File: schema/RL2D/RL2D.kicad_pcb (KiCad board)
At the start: 2 copper layers, 9 parts, among them J1 Steer_Joystick, SW1 SW_FancyButton, SW2 SW_FancyButton, SW3 SW_FancyButton, SW4 SW_On, U1 ILI9341 2.8" TFT LCD

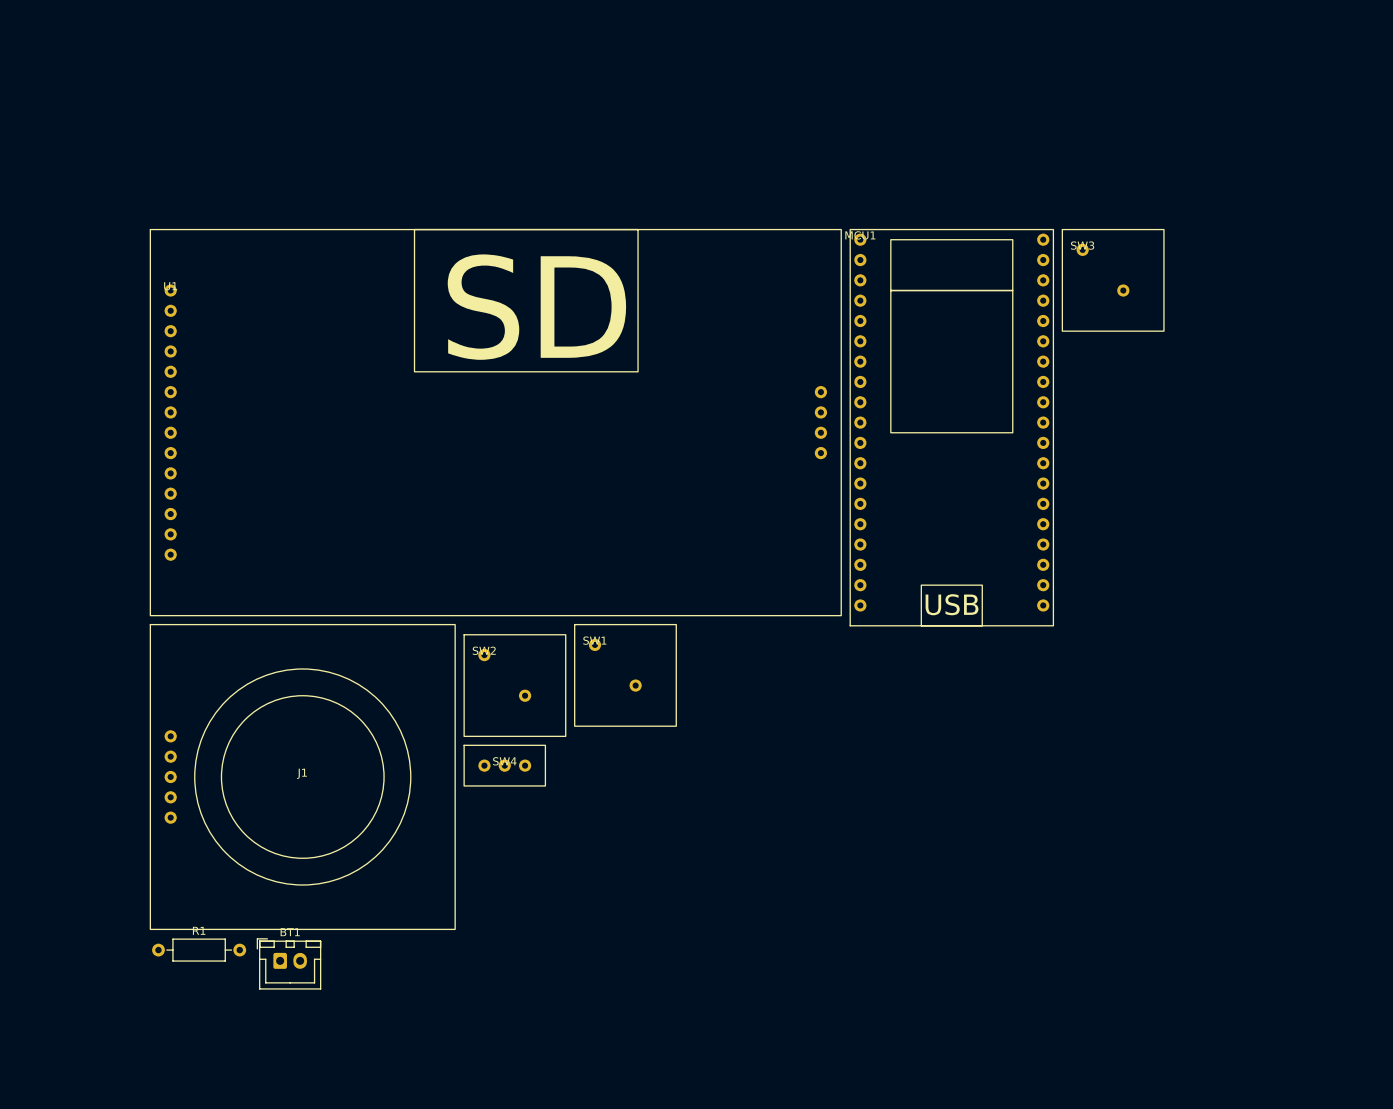
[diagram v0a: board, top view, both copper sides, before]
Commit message: newpcb
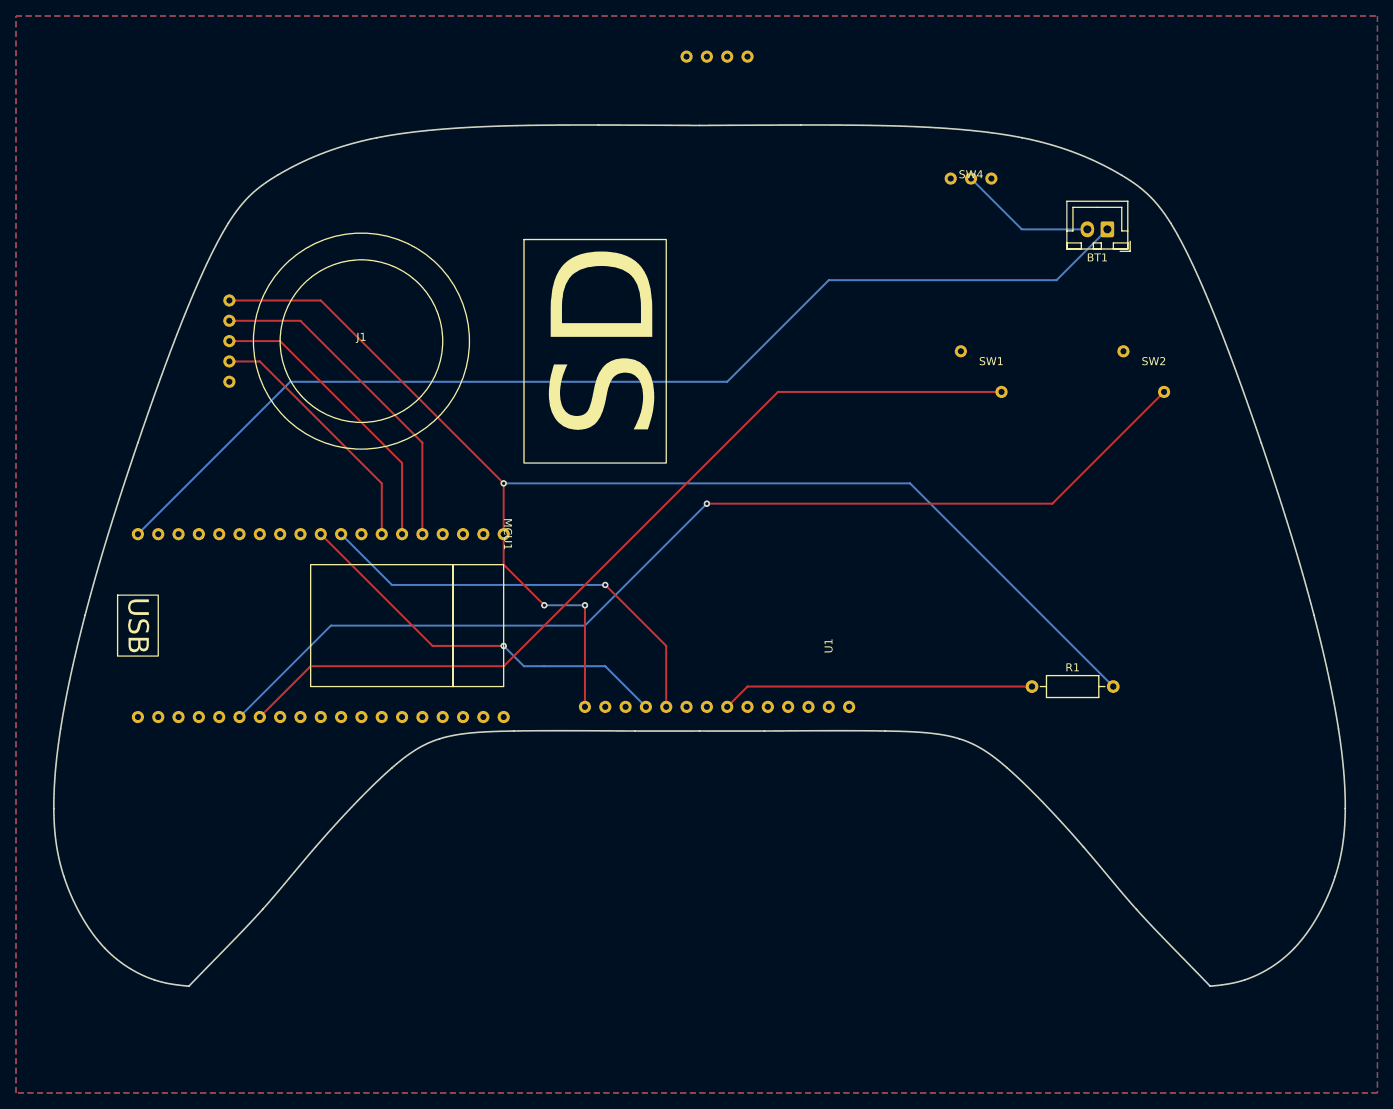
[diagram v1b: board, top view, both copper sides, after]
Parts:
- removed SW3: SW_FancyButton, RL2D:FancyButton
- SW1: value SW_FancyButton -> Brake Button
- SW2: value SW_FancyButton -> Accel Button
- SW4: value SW_On -> On Switch
- moved BT1 138.0 mm to (197.4, 47.0), turned to 180 degrees
- moved R1 114.1 mm to (188.0, 104.1)
- moved SW4 93.7 mm to (180.3, 40.6)
- moved SW2 88.4 mm to (199.4, 62.2)
- moved U1 73.4 mm to (132.1, 106.7), turned to 90 degrees
- moved SW1 58.6 mm to (179.1, 62.2)
- moved MCU1 57.8 mm to (121.9, 85.1), turned to -90 degrees
- moved J1 55.0 mm to (104.1, 61.0)
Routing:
- net +3V3: track 0.00 -> 165.6 mm, vias 0 -> 3
- net VDC: track 0.00 -> 137.0 mm
- net Net-(MCU1-Pad25): track 0.00 -> 132.4 mm, vias 0 -> 1
- net Net-(MCU1-Pad26): track 0.00 -> 109.5 mm
- net Net-(MCU1-Pad9): track 0.00 -> 54.0 mm, vias 0 -> 1
- net Net-(MCU1-Pad10): track 0.00 -> 49.6 mm, vias 0 -> 1
- net Net-(J1-Pad2): track 0.00 -> 41.9 mm
- net Net-(R1-Pad1): track 0.00 -> 39.2 mm
- net Net-(J1-Pad3): track 0.00 -> 36.8 mm
- net Net-(J1-Pad4): track 0.00 -> 31.7 mm
- net Net-(BT1-Pad2): track 0.00 -> 17.2 mm
- added copper zone on B.Cu, net GND
- added copper zone on F.Cu, net GND
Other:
- board outline added: 161.4 x 107.6 mm
